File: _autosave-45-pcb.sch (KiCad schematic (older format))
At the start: 28 parts, among them SW1 SW_Push, U1 ATmega32U4-AU, Y1 16MHz

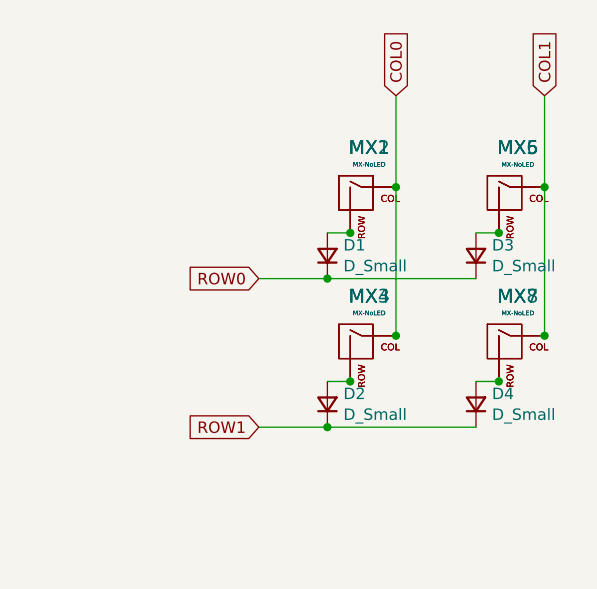
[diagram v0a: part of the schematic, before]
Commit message: Components Placed
Routing Start
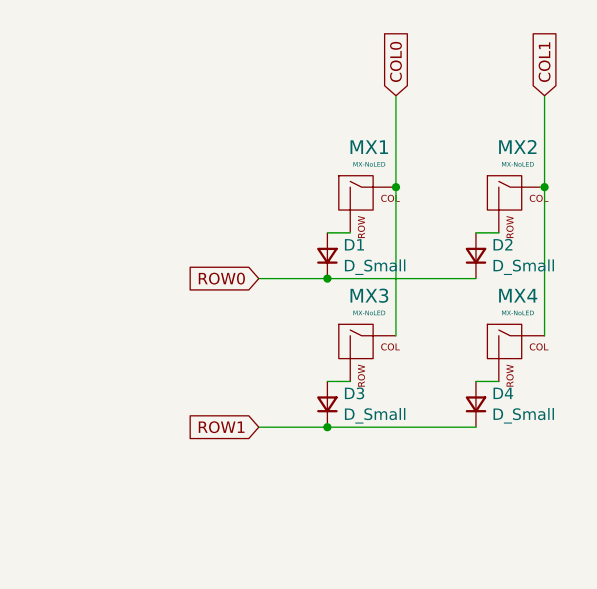
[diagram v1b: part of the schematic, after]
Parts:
- removed D2: D_Small, symbol Device:D_Small
- removed MX2, MX4, MX6, MX8: MX-NoLED, symbol MX_Alps_Hybrid:MX-NoLED
- added D3: D_Small, Diode_SMD:D_SOD-123, symbol Device:D_Small
- C1, C2, C3, C4, C5, C6, C7: footprint (none) -> Capacitor_SMD:C_0805_2012Metric
- D1, D4: footprint (none) -> Diode_SMD:D_SOD-123
- D2: renamed from D3; footprint (none) -> Diode_SMD:D_SOD-123
- F1: footprint (none) -> Fuse:Fuse_1206_3216Metric
- MX1, MX3: footprint (none) -> MX_Alps_Hybrid:MX-1U
- MX2: renamed from MX5; footprint (none) -> MX_Alps_Hybrid:MX-1U
- MX4: renamed from MX7; footprint (none) -> MX_Alps_Hybrid:MX-1U
- R1, R2, R3, R4: footprint (none) -> Resistor_SMD:R_0805_2012Metric
- SW1: footprint (none) -> random-keyboard-parts:SKQG-1155865
- USB1: footprint (none) -> random-keyboard-parts:Molex-0548190589
- Y1: footprint (none) -> Crystal:Crystal_SMD_3225-4Pin_3.2x2.5mm
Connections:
- net ROW1: now also D3.1 (K)
- net at MX3.2 (ROW): now also D3.2 (A)
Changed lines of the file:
@@
 F 0 "R4" V 5454 4850 50  0000 C CNN
 F 1 "10k" V 5545 4850 50  0000 C CNN
-F 2 "" H 5650 4850 50  0001 C CNN
+F 2 "Resistor_SMD:R_0805_2012Metric" H 5650 4850 50  0001 C CNN
 F 3 "~" H 5650 4850 50  0001 C CNN
 	1    5650 4850
@@
 F 0 "R2" V 3204 3750 50  0000 C CNN
 F 1 "22" V 3295 3750 50  0000 C CNN
-F 2 "" H 3400 3750 50  0001 C CNN
+F 2 "Resistor_SMD:R_0805_2012Metric" H 3400 3750 50  0001 C CNN
 F 3 "~" H 3400 3750 50  0001 C CNN
 	1    3400 3750
@@
 F 0 "R1" V 2854 3850 50  0000 C CNN
 F 1 "22" V 2945 3850 50  0000 C CNN
-F 2 "" H 3050 3850 50  0001 C CNN
+F 2 "Resistor_SMD:R_0805_2012Metric" H 3050 3850 50  0001 C CNN
 F 3 "~" H 3050 3850 50  0001 C CNN
 	1    3050 3850
@@
 F 0 "C7" H 3392 4246 50  0000 L CNN
 F 1 "1uF" H 3392 4155 50  0000 L CNN
-F 2 "" H 3300 4200 50  0001 C CNN
+F 2 "Capacitor_SMD:C_0805_2012Metric" H 3300 4200 50  0001 C CNN
 F 3 "~" H 3300 4200 50  0001 C CNN
 	1    3300 4200
@@
 F 0 "C1" H 2142 5146 50  0000 L CNN
 F 1 "0.1uF" H 2142 5055 50  0000 L CNN
-F 2 "" H 2050 5100 50  0001 C CNN
+F 2 "Capacitor_SMD:C_0805_2012Metric" H 2050 5100 50  0001 C CNN
 F 3 "~" H 2050 5100 50  0001 C CNN
 	1    2050 5100
@@
 F 0 "C2" H 2542 5146 50  0000 L CNN
 F 1 "0.1uF" H 2542 5055 50  0000 L CNN
-F 2 "" H 2450 5100 50  0001 C CNN
+F 2 "Capacitor_SMD:C_0805_2012Metric" H 2450 5100 50  0001 C CNN
 F 3 "~" H 2450 5100 50  0001 C CNN
 	1    2450 5100
@@
 F 0 "C3" H 2942 5146 50  0000 L CNN
 F 1 "0.1uF" H 2942 5055 50  0000 L CNN
-F 2 "" H 2850 5100 50  0001 C CNN
+F 2 "Capacitor_SMD:C_0805_2012Metric" H 2850 5100 50  0001 C CNN
 F 3 "~" H 2850 5100 50  0001 C CNN
 	1    2850 5100
@@
 F 0 "C6" H 3342 5146 50  0000 L CNN
 F 1 "10uF" H 3342 5055 50  0000 L CNN
-F 2 "" H 3250 5100 50  0001 C CNN
+F 2 "Capacitor_SMD:C_0805_2012Metric" H 3250 5100 50  0001 C CNN
 F 3 "~" H 3250 5100 50  0001 C CNN
 	1    3250 5100
@@
 F 0 "Y1" V 3304 3194 50  0000 L CNN
 F 1 "16MHz" V 3395 3194 50  0000 L CNN
-F 2 "" H 3350 3050 50  0001 C CNN
+F 2 "Crystal:Crystal_SMD_3225-4Pin_3.2x2.5mm" H 3350 3050 50  0001 C CNN
 F 3 "~" H 3350 3050 50  0001 C CNN
 	1    3350 3050
@@
 F 0 "C4" V 2821 2900 50  0000 C CNN
 F 1 "22pF" V 2912 2900 50  0000 C CNN
-F 2 "" H 3050 2900 50  0001 C CNN
+F 2 "Capacitor_SMD:C_0805_2012Metric" H 3050 2900 50  0001 C CNN
 F 3 "~" H 3050 2900 50  0001 C CNN
 	1    3050 2900
@@
 F 0 "C5" V 2821 3250 50  0000 C CNN
 F 1 "22pF" V 2912 3250 50  0000 C CNN
-F 2 "" H 3050 3250 50  0001 C CNN
+F 2 "Capacitor_SMD:C_0805_2012Metric" H 3050 3250 50  0001 C CNN
 F 3 "~" H 3050 3250 50  0001 C CNN
 	1    3050 3250
@@
 F 0 "SW1" H 3600 2735 50  0000 C CNN
 F 1 "SW_Push" H 3600 2644 50  0000 C CNN
-F 2 "" H 3600 2650 50  0001 C CNN
+F 2 "random-keyboard-parts:SKQG-1155865" H 3600 2650 50  0001 C CNN
 F 3 "~" H 3600 2650 50  0001 C CNN
 	1    3600 2450
@@
 F 0 "R3" H 3859 2246 50  0000 L CNN
 F 1 "10k" H 3859 2155 50  0000 L CNN
-F 2 "" H 3800 2200 50  0001 C CNN
+F 2 "Resistor_SMD:R_0805_2012Metric" H 3800 2200 50  0001 C CNN
 F 3 "~" H 3800 2200 50  0001 C CNN
 	1    3800 2200
@@
 F 0 "USB1" V 1437 1567 60  0000 C CNN
 F 1 "Molex-0548190589" V 1331 1567 60  0000 C CNN
-F 2 "" H 900 1600 60  0001 C CNN
+F 2 "random-keyboard-parts:Molex-0548190589" H 900 1600 60  0001 C CNN
 F 3 "" H 900 1600 60  0001 C CNN
 	1    900  1600
@@
 F 0 "F1" V 1495 1400 50  0000 C CNN
 F 1 "500mA" V 1586 1400 50  0000 C CNN
-F 2 "" H 1750 1200 50  0001 L CNN
+F 2 "Fuse:Fuse_1206_3216Metric" H 1750 1200 50  0001 L CNN
 F 3 "~" H 1700 1400 50  0001 C CNN
 	1    1700 1400
@@
 F 0 "MX1" H 7083 1573 60  0000 C CNN
 F 1 "MX-NoLED" H 7083 1499 20  0000 C CNN
-F 2 "" H 6425 1325 60  0001 C CNN
+F 2 "MX_Alps_Hybrid:MX-1U" H 6425 1325 60  0001 C CNN
 F 3 "" H 6425 1325 60  0001 C CNN
 	1    7050 1350
@@
 F 0 "D1" V 6946 1530 50  0000 R CNN
 F 1 "D_Small" V 6855 1530 50  0000 R CNN
-F 2 "" V 6900 1600 50  0001 C CNN
+F 2 "Diode_SMD:D_SOD-123" V 6900 1600 50  0001 C CNN
 F 3 "~" V 6900 1600 50  0001 C CNN
 	1    6900 1600
@@
 $Comp
 L MX_Alps_Hybrid:MX-NoLED MX2
-U 1 1 5EF56C9D
-P 7050 1350
-F 0 "MX2" H 7083 1573 60  0000 C CNN
-F 1 "MX-NoLED" H 7083 1499 20  0000 C CNN
-F 2 "" H 6425 1325 60  0001 C CNN
-F 3 "" H 6425 1325 60  0001 C CNN
-	1    7050 1350
-	1    0    0    -1
-$EndComp
-Connection ~ 7000 1500
-$Comp
-L MX_Alps_Hybrid:MX-NoLED MX5
 U 1 1 5EF62352
 P 7700 1350
-F 0 "MX5" H 7733 1573 60  0000 C CNN
+F 0 "MX2" H 7733 1573 60  0000 C CNN
 F 1 "MX-NoLED" H 7733 1499 20  0000 C CNN
-F 2 "" H 7075 1325 60  0001 C CNN
+F 2 "MX_Alps_Hybrid:MX-1U" H 7075 1325 60  0001 C CNN
 F 3 "" H 7075 1325 60  0001 C CNN
 	1    7700 1350
@@
 $EndComp
 $Comp
-L Device:D_Small D3
+L Device:D_Small D2
 U 1 1 5EF62358
 P 7550 1600
-F 0 "D3" V 7596 1530 50  0000 R CNN
+F 0 "D2" V 7596 1530 50  0000 R CNN
 F 1 "D_Small" V 7505 1530 50  0000 R CNN
-F 2 "" V 7550 1600 50  0001 C CNN
+F 2 "Diode_SMD:D_SOD-123" V 7550 1600 50  0001 C CNN
 F 3 "~" V 7550 1600 50  0001 C CNN
 	1    7550 1600
@@
 Wire Wire Line
 	7650 1500 7550 1500
-$Comp
-L MX_Alps_Hybrid:MX-NoLED MX6
-U 1 1 5EF6235F
-P 7700 1350
-F 0 "MX6" H 7733 1573 60  0000 C CNN
-F 1 "MX-NoLED" H 7733 1499 20  0000 C CNN
-F 2 "" H 7075 1325 60  0001 C CNN
-F 3 "" H 7075 1325 60  0001 C CNN
-	1    7700 1350
-	1    0    0    -1
-$EndComp
-Connection ~ 7650 1500
 $Comp
 L MX_Alps_Hybrid:MX-NoLED MX3
@@
 F 0 "MX3" H 7083 2223 60  0000 C CNN
 F 1 "MX-NoLED" H 7083 2149 20  0000 C CNN
-F 2 "" H 6425 1975 60  0001 C CNN
+F 2 "MX_Alps_Hybrid:MX-1U" H 6425 1975 60  0001 C CNN
 F 3 "" H 6425 1975 60  0001 C CNN
 	1    7050 2000
 	1    0    0    -1
 $EndComp
-$Comp
-L Device:D_Small D2
-U 1 1 5EF6520E
-P 6900 2250
-F 0 "D2" V 6946 2180 50  0000 R CNN
-F 1 "D_Small" V 6855 2180 50  0000 R CNN
-F 2 "" V 6900 2250 50  0001 C CNN
-F 3 "~" V 6900 2250 50  0001 C CNN
-	1    6900 2250
-	0    -1   -1   0
-$EndComp
 Wire Wire Line
 	7000 2150 6900 2150
 $Comp
 L MX_Alps_Hybrid:MX-NoLED MX4
-U 1 1 5EF65215
-P 7050 2000
-F 0 "MX4" H 7083 2223 60  0000 C CNN
-F 1 "MX-NoLED" H 7083 2149 20  0000 C CNN
-F 2 "" H 6425 1975 60  0001 C CNN
-F 3 "" H 6425 1975 60  0001 C CNN
-	1    7050 2000
-	1    0    0    -1
-$EndComp
-Connection ~ 7000 2150
-$Comp
-L MX_Alps_Hybrid:MX-NoLED MX7
 U 1 1 5EF6655B
 P 7700 2000
-F 0 "MX7" H 7733 2223 60  0000 C CNN
+F 0 "MX4" H 7733 2223 60  0000 C CNN
 F 1 "MX-NoLED" H 7733 2149 20  0000 C CNN
-F 2 "" H 7075 1975 60  0001 C CNN
+F 2 "MX_Alps_Hybrid:MX-1U" H 7075 1975 60  0001 C CNN
 F 3 "" H 7075 1975 60  0001 C CNN
 	1    7700 2000
@@
 F 0 "D4" V 7596 2180 50  0000 R CNN
 F 1 "D_Small" V 7505 2180 50  0000 R CNN
-F 2 "" V 7550 2250 50  0001 C CNN
+F 2 "Diode_SMD:D_SOD-123" V 7550 2250 50  0001 C CNN
 F 3 "~" V 7550 2250 50  0001 C CNN
 	1    7550 2250
@@
 Wire Wire Line
 	7650 2150 7550 2150
-$Comp
-L MX_Alps_Hybrid:MX-NoLED MX8
-U 1 1 5EF66568
-P 7700 2000
-F 0 "MX8" H 7733 2223 60  0000 C CNN
-F 1 "MX-NoLED" H 7733 2149 20  0000 C CNN
-F 2 "" H 7075 1975 60  0001 C CNN
-F 3 "" H 7075 1975 60  0001 C CNN
-	1    7700 2000
-	1    0    0    -1
-$EndComp
-Connection ~ 7650 2150
 Wire Wire Line
 	7200 1950 7200 1300
-Connection ~ 7200 1950
 Connection ~ 7200 1300
 Wire Wire Line
@@
 Wire Wire Line
 	7850 1950 7850 1300
-Connection ~ 7850 1950
 Connection ~ 7850 1300
 Wire Wire Line
 	7850 1300 7850 900
-Wire Wire Line
-	7550 2350 6900 2350
-Connection ~ 6900 2350
-Wire Wire Line
-	6900 2350 6600 2350
 Wire Wire Line
 	7550 1700 6900 1700
@@
 Text GLabel 6600 2350 0    50   Input ~ 0
 ROW1
+Wire Wire Line
+	6600 2350 6900 2350
+$Comp
+L Device:D_Small D3
+U 1 1 5EF8251B
+P 6900 2250
+F 0 "D3" V 6946 2180 50  0000 R CNN
+F 1 "D_Small" V 6855 2180 50  0000 R CNN
+F 2 "Diode_SMD:D_SOD-123" V 6900 2250 50  0001 C CNN
+F 3 "~" V 6900 2250 50  0001 C CNN
+	1    6900 2250
+	0    -1   -1   0
+$EndComp
+Connection ~ 6900 2350
+Wire Wire Line
+	6900 2350 7550 2350
 $EndSCHEMATC

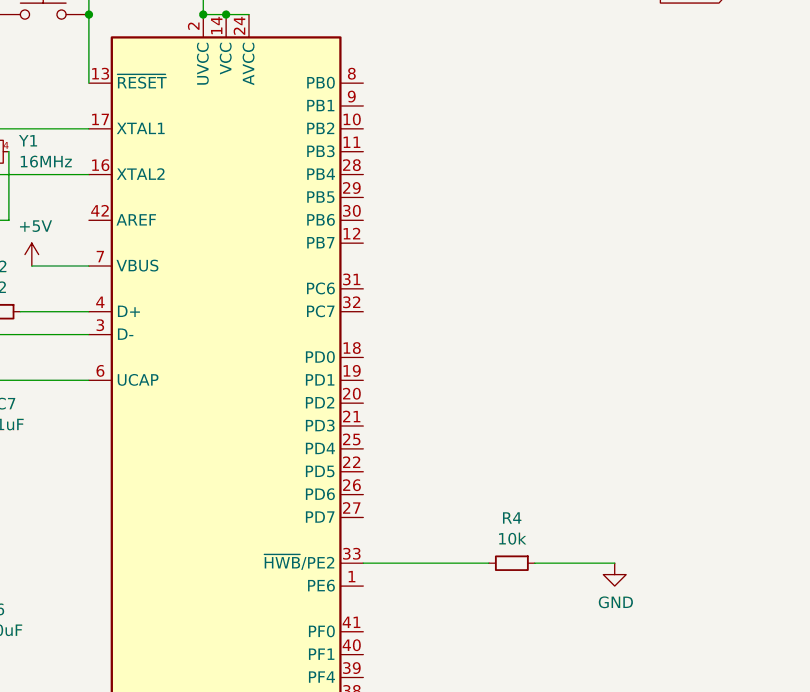
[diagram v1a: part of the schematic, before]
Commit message: Done
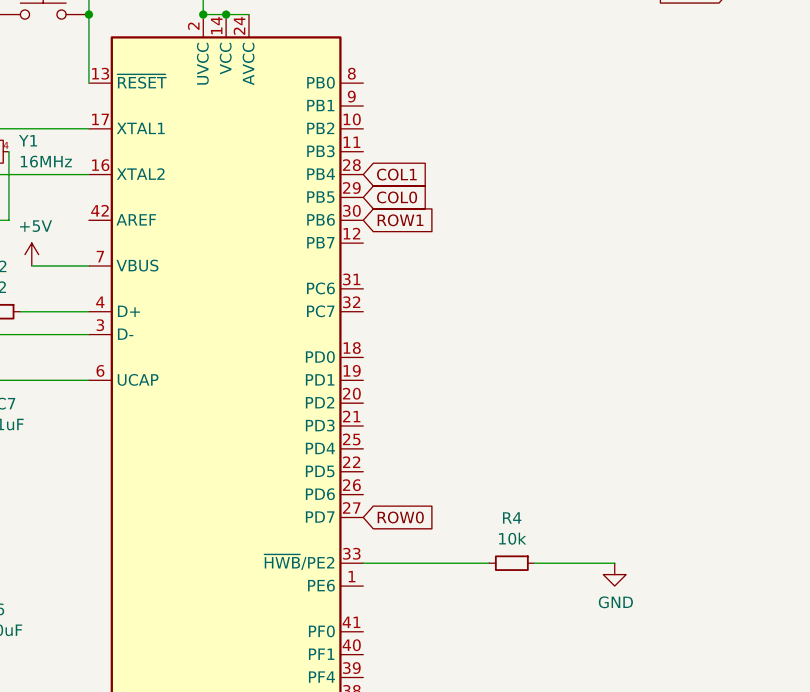
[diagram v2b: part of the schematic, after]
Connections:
- net COL0: now also U1.29 (PB5)
- net COL1: now also U1.28 (PB4)
- net ROW0: now also U1.27 (PD7)
- net ROW1: now also U1.30 (PB6)
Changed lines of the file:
@@
 Wire Wire Line
 	6900 2350 7550 2350
+Text GLabel 5000 3150 2    50   Input ~ 0
+COL1
+Text GLabel 5000 3250 2    50   Input ~ 0
+COL0
+Text GLabel 5000 3350 2    50   Input ~ 0
+ROW1
+Text GLabel 5000 4650 2    50   Input ~ 0
+ROW0
 $EndSCHEMATC
